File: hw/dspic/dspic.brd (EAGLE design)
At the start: 60.6 x 45.7 mm, 23 parts, among them Q1 8MHz, U1 DSPIC33FJ128MC802-I/SP

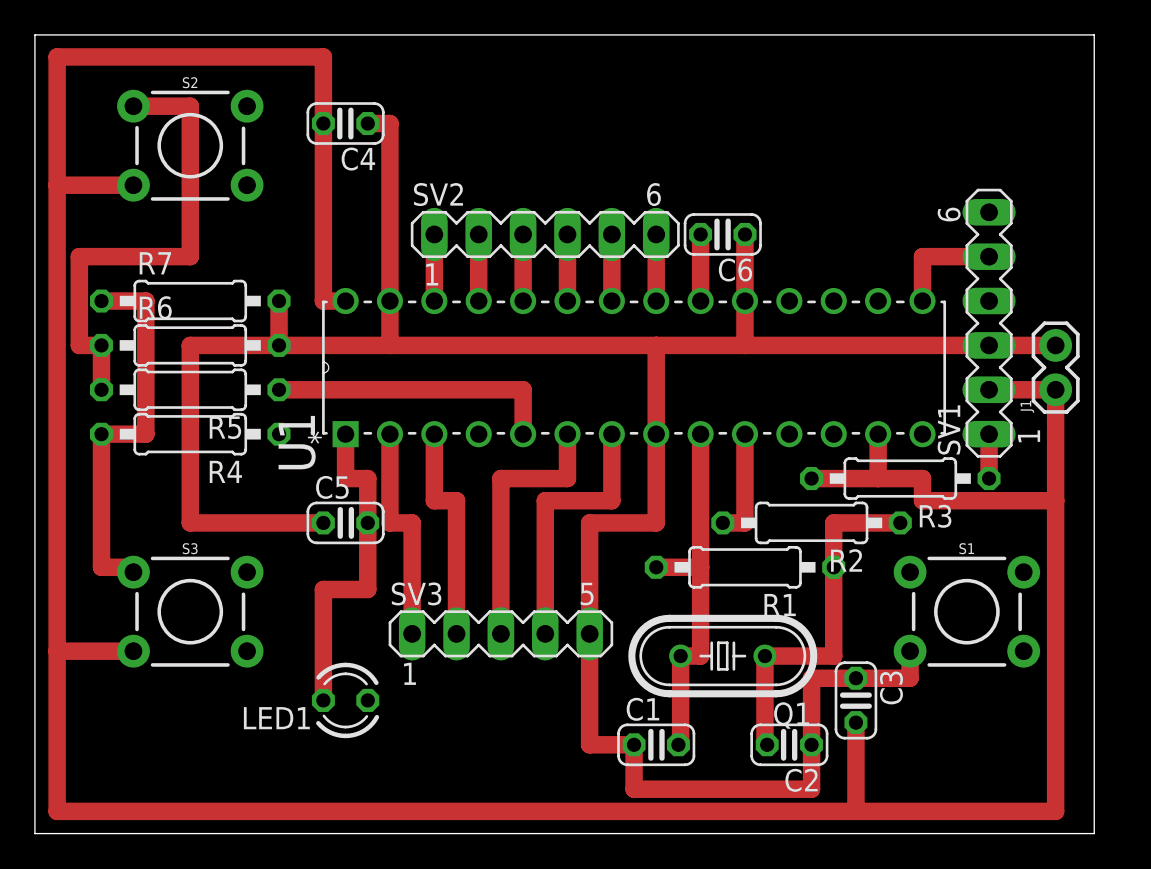
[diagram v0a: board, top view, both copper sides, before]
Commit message: layout
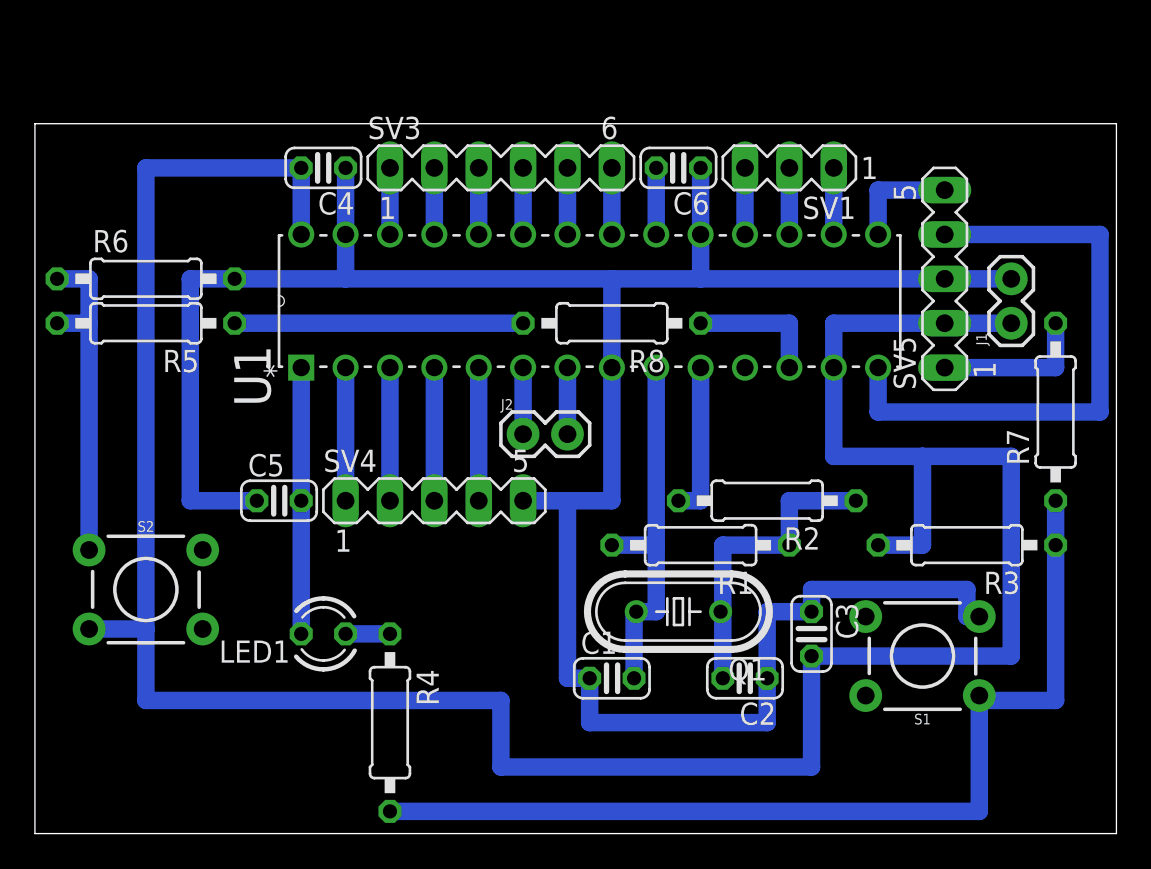
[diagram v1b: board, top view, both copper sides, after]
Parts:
- removed S3: (no value), SparkFun-Switches:TACTILE_SWITCH_PTH_6.0MM
- removed SV2: (no value), con-lstb:MA06-1
- added J2: (no value), SparkFun-Connectors:1X02
- added R8: 0 Jump, resistor:0207/10
- added SV4, SV5: (no value), con-lstb:MA05-1
- R4, R7: value 10K -> 0 Jump
- SV1: device con-lstb:MA06-1 -> con-lstb:MA03-1
- SV3: device con-lstb:MA05-1 -> con-lstb:MA06-1
- moved R7 49.9 mm to (58.4, 24.1), turned to 90 degrees
- moved SV3 26.7 mm to (26.7, 38.1)
- moved S2 25.5 mm to (6.35, 14.0)
- moved R4 20.1 mm to (20.3, 6.35), turned to 270 degrees
- moved SV1 14.5 mm to (43.2, 38.1), turned to 180 degrees
- moved R3 5.39 mm to (53.3, 16.5)
- moved C6 4.58 mm to (36.8, 38.1)
- moved J1 4.58 mm to (55.9, 29.2)
- moved R5 4.58 mm to (6.35, 29.2)
- moved C1 4.58 mm to (33.0, 8.89)
- moved C2 4.58 mm to (40.6, 8.89)
- moved R6 4.58 mm to (6.35, 31.8)
- moved C3 4.58 mm to (44.5, 11.4)
- moved U1 4.58 mm to (31.8, 30.5)
- moved C5 4.02 mm to (14.0, 19.1)
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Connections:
- removed net N$3 (its old number): R4.2, R7.1, S3.1
- new net INT0: SV1.1, U1.16
- new net KEY: R8.1, U1.12
- new net N$4: R3.1, R4.2, R7.1, S1.1
- new net N$5: LED1.A, R4.1
- new net N$6: R5.1, R8.2
- new net U1RX: SV1.2, U1.17
- new net U1TX: SV1.3, U1.18
- net !MCLR!: now also R7.2, SV5.1; no longer LED1.A, R3.1, S1.1, SV1.1
- net +3V3: now also SV5.2; no longer S3.3, SV1.2
- net GND: now also SV4.5, SV5.3; no longer R7.2, SV1.3, SV3.5
- net H1: now also SV3.2; no longer SV2.2
- net H2: now also SV3.4; no longer SV2.4
- net H3: now also SV3.6; no longer SV2.6
- net IMOTORA: now also SV4.3, U1.4; no longer SV3.3, U1.6
- net IMOTORB: now also SV4.1; no longer SV3.1
- net IMOTORBUS: now also SV4.2; no longer SV3.2
- net L1: now also SV3.1; no longer SV2.1
- net L2: now also SV3.3; no longer SV2.3
- net L3: now also SV3.5; no longer SV2.5
- net N$10: now also J2.1, U1.6; no longer R5.1, U1.5
- net N$11: now also J2.2, U1.7; no longer R4.1, U1.4
- net PGEC: now also SV5.5; no longer SV1.5
- net PGED: now also SV5.4; no longer SV1.4
- net POT: now also SV4.4, U1.5; no longer SV3.4, U1.7
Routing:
- net N$4: track 0.00 -> 56.2 mm
- net +3V3: track 190.3 -> 153.1 mm
- net PGED: track 0.00 -> 34.3 mm
- net N$3 (its old number): track 22.4 -> 0.00 mm
- net N$6: track 0.00 -> 16.5 mm
- net N$10: track 16.5 -> 3.81 mm
- net N$3: track 27.1 -> 19.2 mm
- net POT: track 15.2 -> 7.62 mm
- net KEY: track 0.00 -> 7.62 mm
- net IMOTORA: track 15.2 -> 7.62 mm
- net !MCLR!: track 2.54 -> 8.89 mm
- net GND: track 145.6 -> 139.4 mm
- net IMOTORBUS: track 12.7 -> 7.62 mm
- net IMOTORB: track 12.7 -> 7.62 mm
- net U1TX: track 0.00 -> 3.81 mm
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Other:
- board size 60.6 x 45.7 mm -> 61.9 x 40.6 mm
